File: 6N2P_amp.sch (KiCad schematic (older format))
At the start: 83 parts, among them J1 guitar_in, J2 speaker, J3 fx_send, J4 fx_return, J5 foot_sw, U1 ECC83, U2 ECC83, U3 6N1P, U4 DSN-MINI-360, U5 DSN-MINI-360, U6 DSN-MINI-360, U7 NCH6100HV

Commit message: snap
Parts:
- RV1, RV2, RV3, RV4, RV5, RV6: footprint Potentiometer_THT:Potentiometer_Alps_RK163_Single_Horizontal -> Connector_PinHeader_2.54mm:PinHeader_1x03_P2.54mm_Vertical
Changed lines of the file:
@@
 F 0 "RV1" H 7430 9096 50  0000 R CNN
 F 1 "500k log" H 7430 9005 50  0000 R CNN
-F 2 "Potentiometer_THT:Potentiometer_Alps_RK163_Single_Horizontal" H 7500 9050 50  0001 C CNN
+F 2 "Connector_PinHeader_2.54mm:PinHeader_1x03_P2.54mm_Vertical" H 7500 9050 50  0001 C CNN
 F 3 "~" H 7500 9050 50  0001 C CNN
 	1    7500 9050
@@
 F 0 "RV2" H 10780 9096 50  0000 R CNN
 F 1 "500k log" H 10780 9005 50  0000 R CNN
-F 2 "Potentiometer_THT:Potentiometer_Alps_RK163_Single_Horizontal" H 10850 9050 50  0001 C CNN
+F 2 "Connector_PinHeader_2.54mm:PinHeader_1x03_P2.54mm_Vertical" H 10850 9050 50  0001 C CNN
 F 3 "~" H 10850 9050 50  0001 C CNN
 	1    10850 9050
@@
 F 0 "RV5" H 17230 9146 50  0000 R CNN
 F 1 "50k lin" H 17230 9055 50  0000 R CNN
-F 2 "Potentiometer_THT:Potentiometer_Alps_RK163_Single_Horizontal" H 17300 9100 50  0001 C CNN
+F 2 "Connector_PinHeader_2.54mm:PinHeader_1x03_P2.54mm_Vertical" H 17300 9100 50  0001 C CNN
 F 3 "~" H 17300 9100 50  0001 C CNN
 	1    17300 9100
@@
 F 0 "RV4" H 17230 8546 50  0000 R CNN
 F 1 "500k log" H 17230 8455 50  0000 R CNN
-F 2 "Potentiometer_THT:Potentiometer_Alps_RK163_Single_Horizontal" H 17300 8500 50  0001 C CNN
+F 2 "Connector_PinHeader_2.54mm:PinHeader_1x03_P2.54mm_Vertical" H 17300 8500 50  0001 C CNN
 F 3 "~" H 17300 8500 50  0001 C CNN
 	1    17300 8500
@@
 F 0 "RV3" H 17231 7946 50  0000 R CNN
 F 1 "250k lin" H 17231 7855 50  0000 R CNN
-F 2 "Potentiometer_THT:Potentiometer_Alps_RK163_Single_Horizontal" H 17300 7900 50  0001 C CNN
+F 2 "Connector_PinHeader_2.54mm:PinHeader_1x03_P2.54mm_Vertical" H 17300 7900 50  0001 C CNN
 F 3 "~" H 17300 7900 50  0001 C CNN
 	1    17300 7900
@@
 F 0 "RV6" H 18030 8546 50  0000 R CNN
 F 1 "1M log" H 18030 8455 50  0000 R CNN
-F 2 "Potentiometer_THT:Potentiometer_Alps_RK163_Single_Horizontal" H 18100 8500 50  0001 C CNN
+F 2 "Connector_PinHeader_2.54mm:PinHeader_1x03_P2.54mm_Vertical" H 18100 8500 50  0001 C CNN
 F 3 "~" H 18100 8500 50  0001 C CNN
 	1    18100 8500

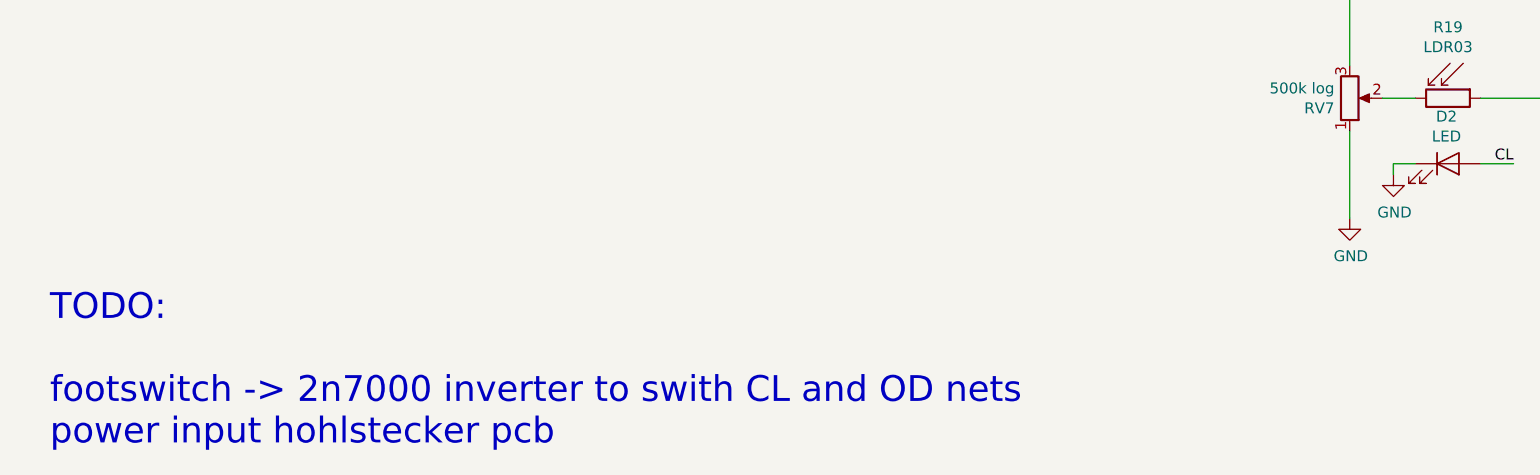
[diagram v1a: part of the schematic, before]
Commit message: new evening
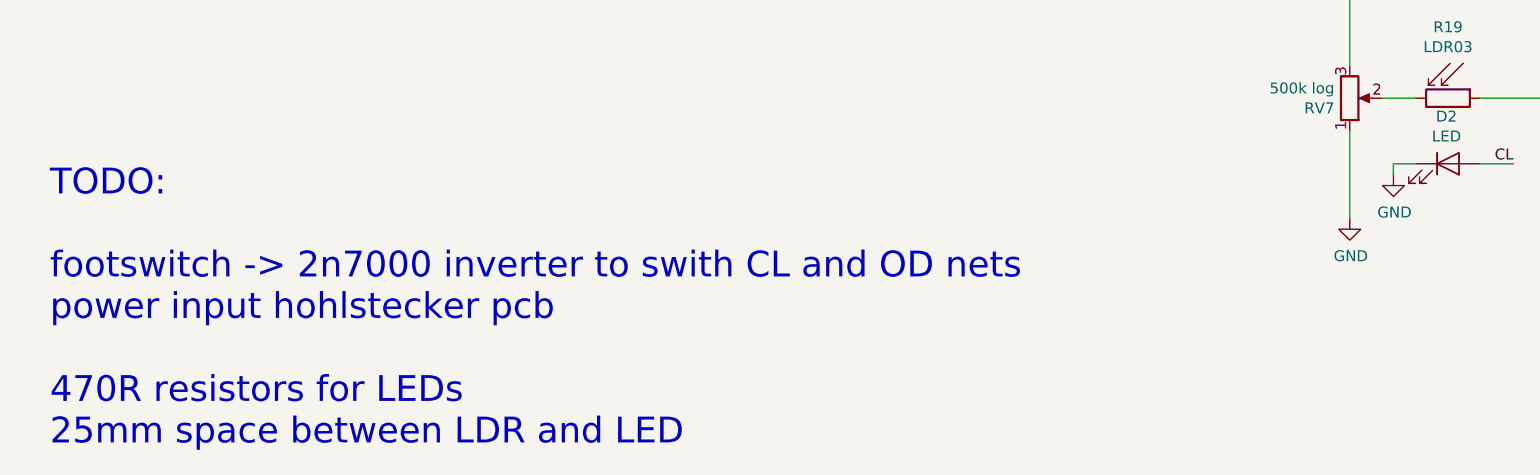
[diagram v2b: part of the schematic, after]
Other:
- note added: "TODO:\n\nfootswitch -> 2n7000 inverter to swith CL and OD nets\npower input hohlstecker pcb\n\n470R resistors for LEDs\n25mm space between LDR and LED"
- note removed: "TODO:\n\nfootswitch -> 2n7000 inverter to swith CL and OD nets\npower input hohlstecker pcb"
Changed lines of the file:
@@
 	12900 8500 12900 8450
 Text Notes 1550 13600 0    118  ~ 0
-TODO:\n\nfootswitch -> 2n7000 inverter to swith CL and OD nets\npower input hohlstecker pcb
+TODO:\n\nfootswitch -> 2n7000 inverter to swith CL and OD nets\npower input hohlstecker pcb\n\n470R resistors for LEDs\n25mm space between LDR and LED
 $Comp
 L micha_custom:6.3MMTRSSwitched J5
